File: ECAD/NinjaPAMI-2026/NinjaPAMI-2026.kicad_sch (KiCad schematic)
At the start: 76 parts, among them J1 Con_Batt, J10 CON_EV_01, J11 Conn_01x04, J12 OLED, J13 RightMotor, J14 LeftMotor, J2 Servo, J3 Servo, J4 Sensor_RIGHT, J5 Sensor_Center, J6 Sensor_LEFT, J7 CON_EV_02, J8 CON_EV_02, J9 CON_PUMP_01, Q1 AO3400A, Q2 AO3400A, Q3 AO3400A, Q4 AO3400A, SW1 SW_SPDT, SW2 SW_Reed, SW3 SW_SPDT, U1 R-78E5.0-1.0, U2 XIAO-HALF-HOLE-23P, U3 TMC2209_SILENTSTEPSTICK, U4 TMC2209_SILENTSTEPSTICK

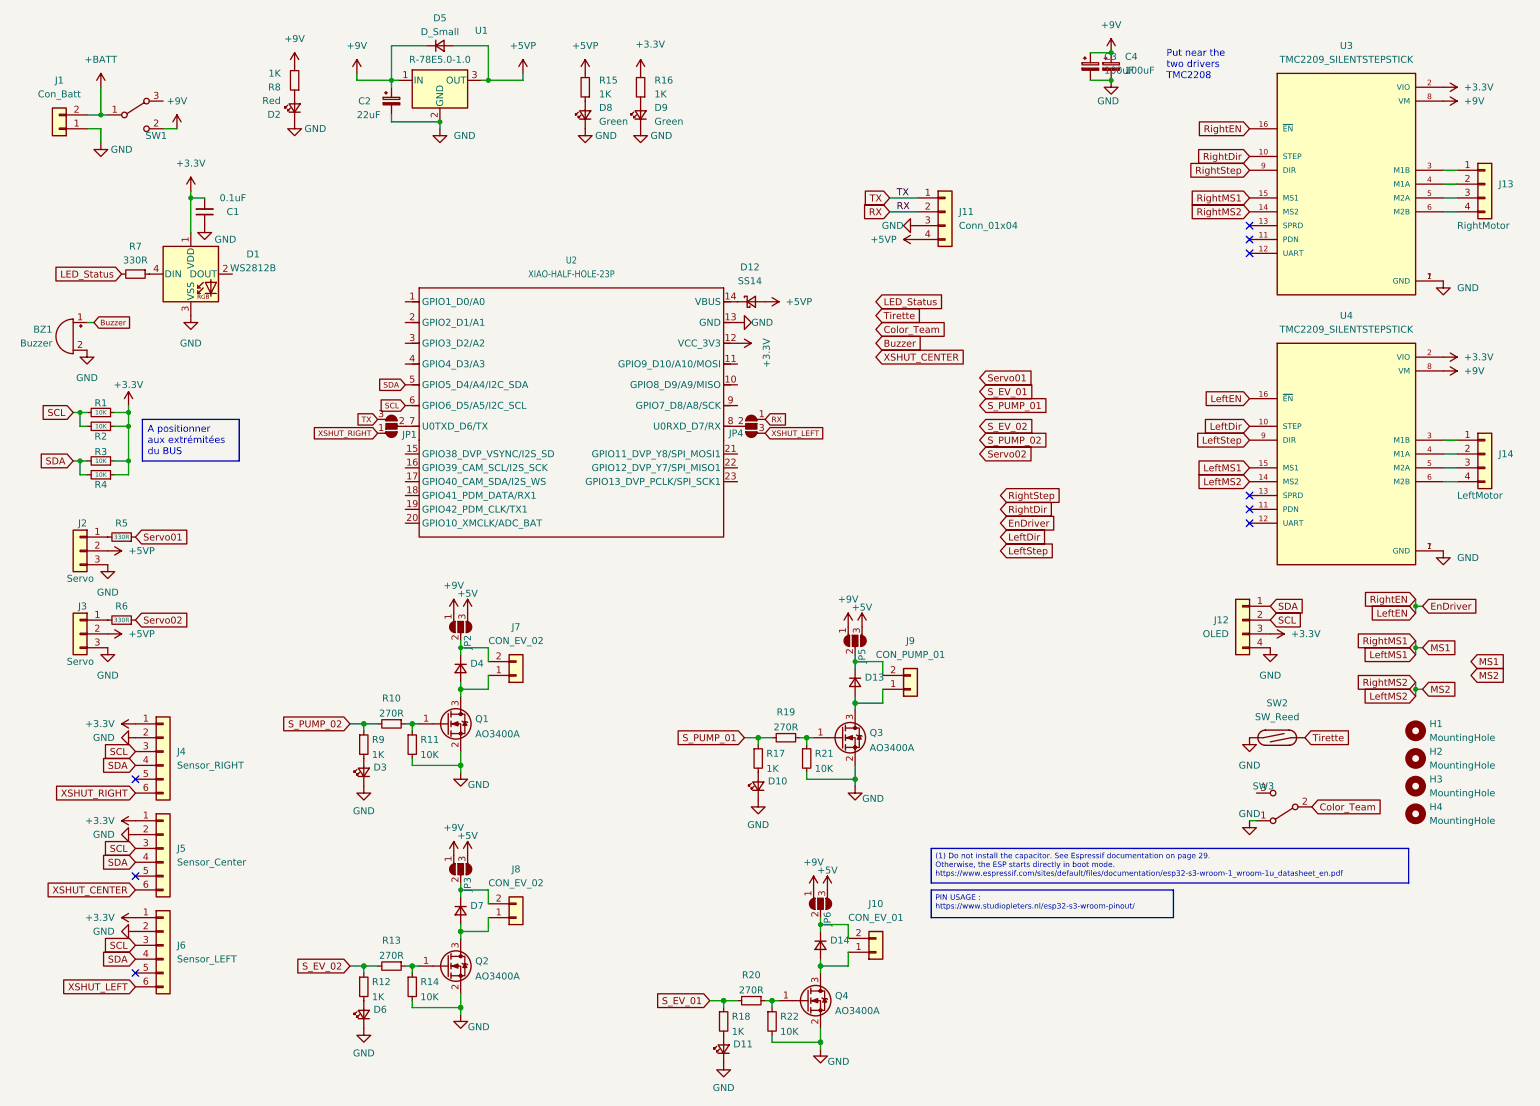
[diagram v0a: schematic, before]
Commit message: placement pump and ev
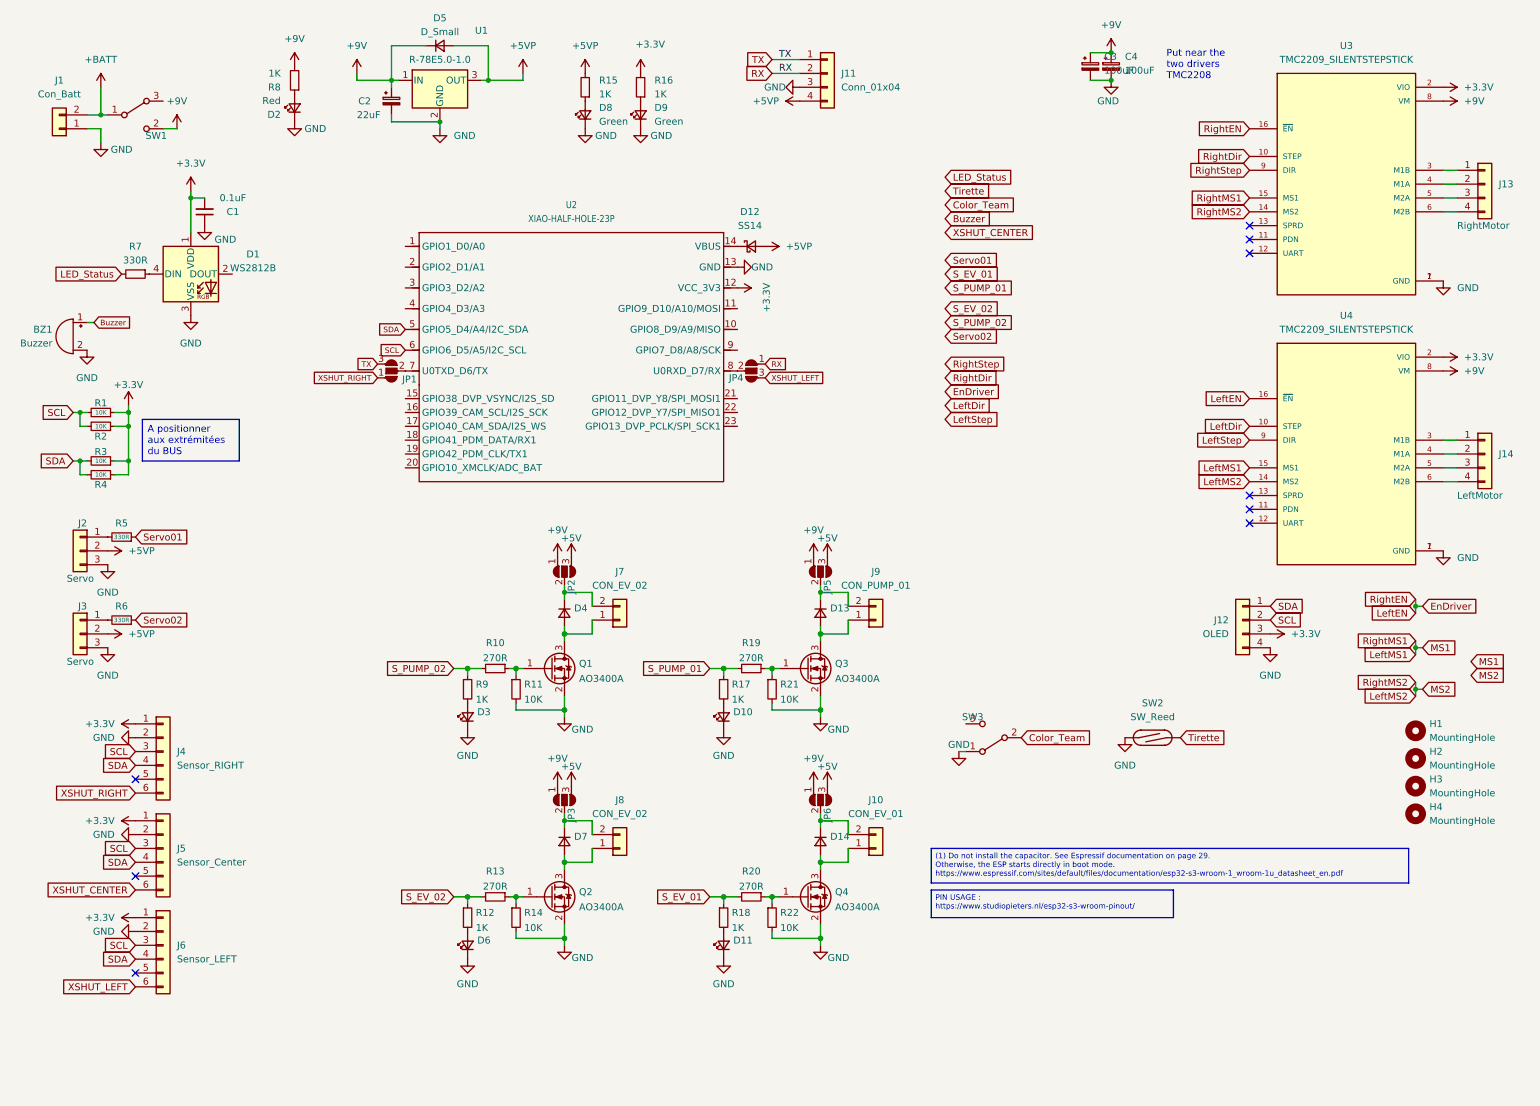
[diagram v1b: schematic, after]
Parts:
- J12: footprint Connector_PinSocket_2.54mm:PinSocket_1x04_P2.54mm_Vertical -> Connector_Molex:Molex_KK-254_AE-6410-04A_1x04_P2.54mm_Vertical
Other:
- moved on the sheet: D10, D11, D12, D13, D14, D3, D4, D6, D7, J10, J11, J7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
